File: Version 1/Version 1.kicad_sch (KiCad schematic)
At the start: 73 parts, among them J1 Conn_01x05, Q1 IPP015N04NF2SAKMA1, Q2 IPP015N04NF2SAKMA1, Q3 IPP015N04NF2SAKMA1, Q4 IPP015N04NF2SAKMA1, Q5 IPP015N04NF2SAKMA1, Q6 IPP015N04NF2SAKMA1, U0 YAAJ_BlackPill_SWD_Breakout, U1 TPS62932, U2 TPS62932, U3 TPS62932, U4 IRS2004, U5 IRS2004, U6 IRS2004

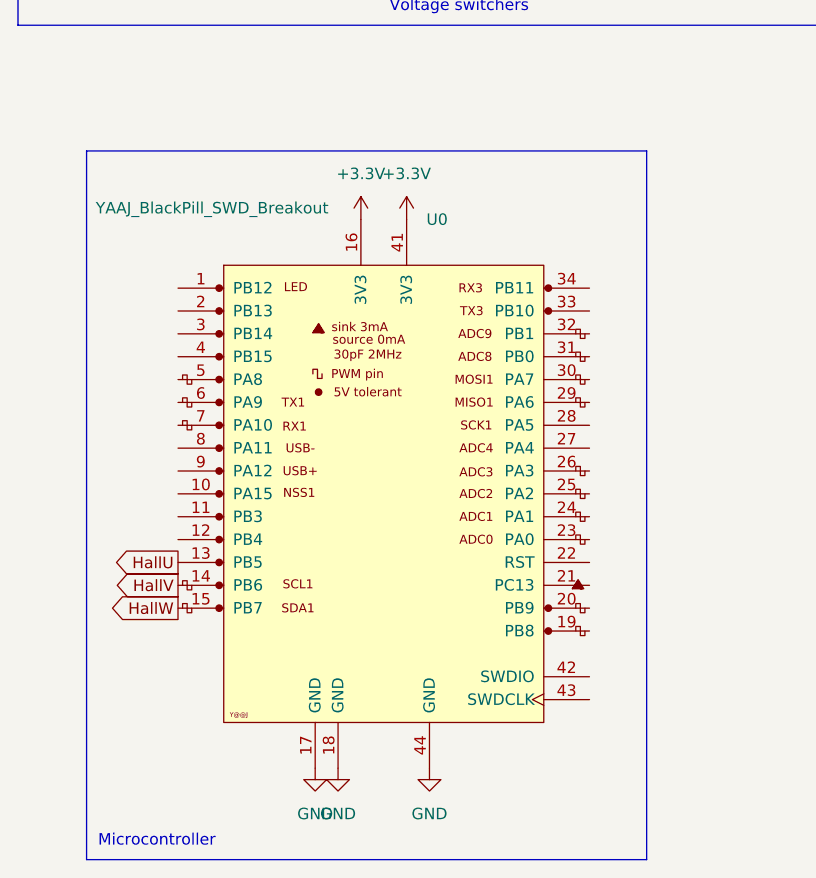
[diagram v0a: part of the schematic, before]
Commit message: updated schem
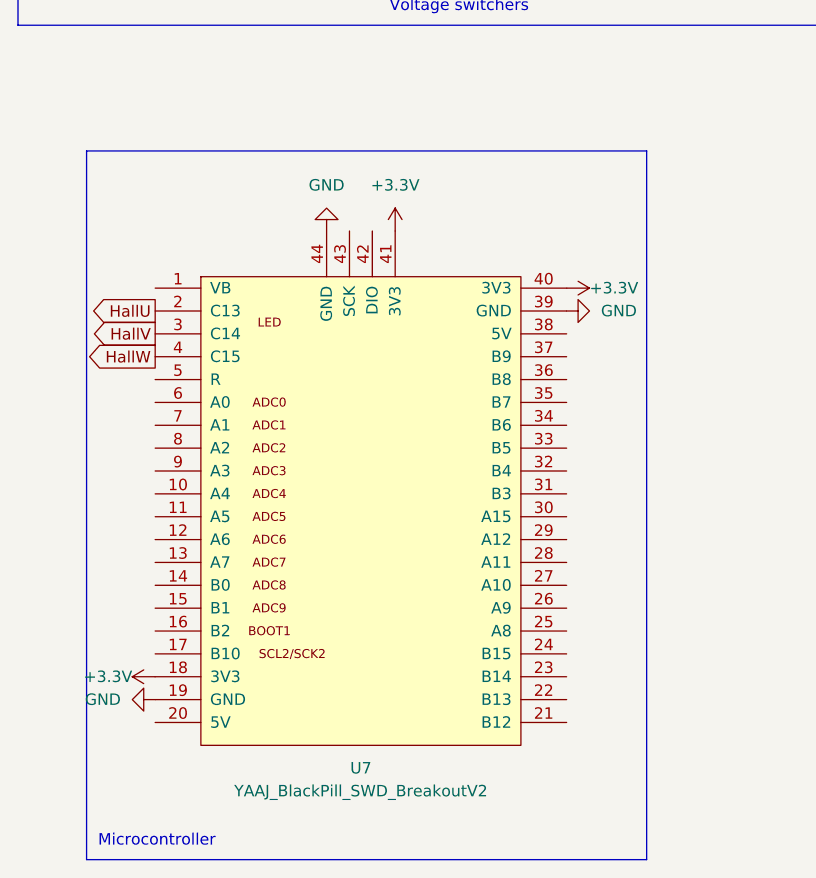
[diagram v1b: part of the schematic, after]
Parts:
- removed U0: YAAJ_BlackPill_SWD_Breakout, Footprints:YAAJ_BlackPill_SWD_1, symbol YAAJ_BlackPill_SWD_Breakout:YAAJ_BlackPill_SWD_Breakout
- added U7: YAAJ_BlackPill_SWD_BreakoutV2, STM32:Blackpill, symbol YAAJ_BlackPill_SWD_BreakoutV2:YAAJ_BlackPill_SWD_BreakoutV2
- C1, C2, C3, C4, C6, C8: footprint (none) -> Capacitor_THT:C_Disc_D3.4mm_W2.1mm_P2.50mm
- C5, C7, C9: footprint (none) -> Capacitor_THT:CP_Radial_D5.0mm_P2.50mm
- L1, L2, L3: footprint IND_MULTICOMP_MCSCH895_MTC -> Inductor_THT:L_Axial_L13.0mm_D4.5mm_P7.62mm_Vertical_Fastron_HCCC
- Q1, Q2, Q3, Q4, Q5, Q6: footprint TO254P475X1028X1996-3P -> LIB_IPP015N04NF2SAKMA1:TO254P475X1028X1996-3P
- R10, R11, R12, R13, R14, R15, R16, R17, R18, R4, R5, R6, R7, R8, R9: footprint (none) -> Resistor_THT:R_Axial_DIN0207_L6.3mm_D2.5mm_P10.16mm_Horizontal
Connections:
- net +3.3V: now also U7.18 (3V3), U7.40 (3V3), U7.41 (3V3)
- net GND: now also U7.19 (GND), U7.39 (GND), U7.44 (GND)
- net HallU: now also U7.2 (C13)
- net HallV: now also U7.3 (C14)
- net HallW: now also U7.4 (C15)
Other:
- company: (none) -> ALSET
- title: (none) -> Motor driver
